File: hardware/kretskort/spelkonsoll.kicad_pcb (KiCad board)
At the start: 2 copper layers, 176.6 x 56.6 mm, 19 parts, among them J1 USB_C_Receptacle_USB2.0, SW1 SW_Push, SW10 SW_Push, SW11 SW_Push, SW12 SW_Push, SW2 SW_Push, SW3 SW_Push, SW4 SW_Push, SW5 SW_Push, SW6 SW_Push, SW7 SW_Push, SW8 SW_Push, SW9 SW_Push, U1 BQ24202DGN, U2 ESP32-DEVKITC-32D, U3 ILI9488

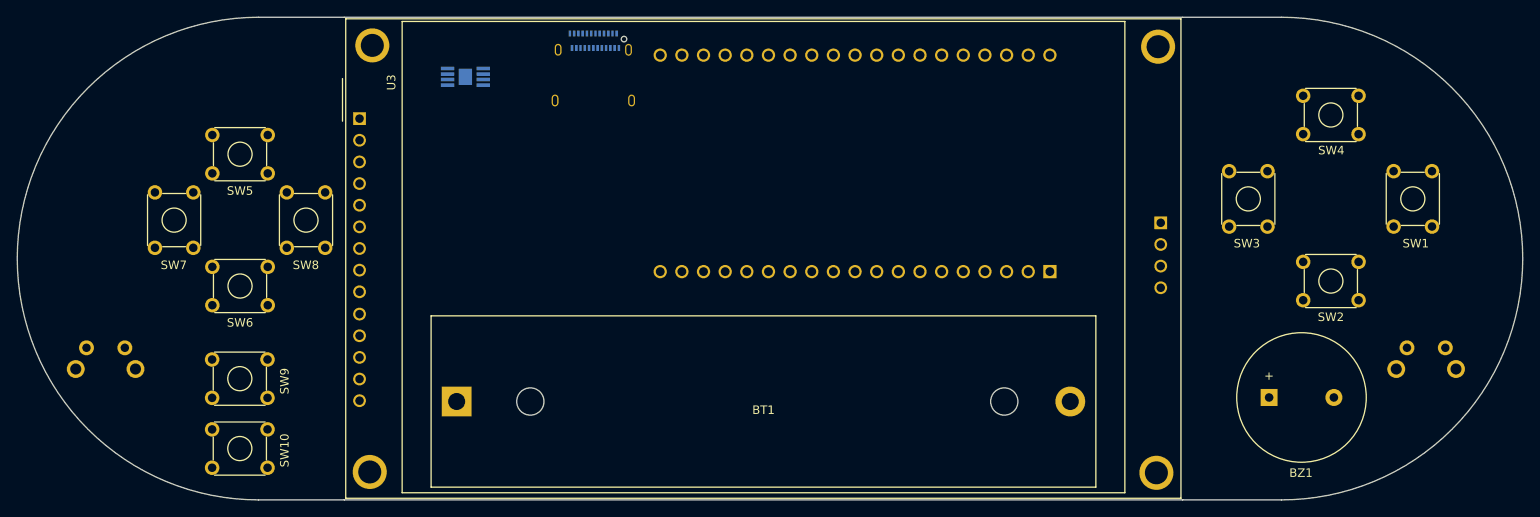
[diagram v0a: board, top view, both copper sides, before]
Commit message: lol glemte å lagre
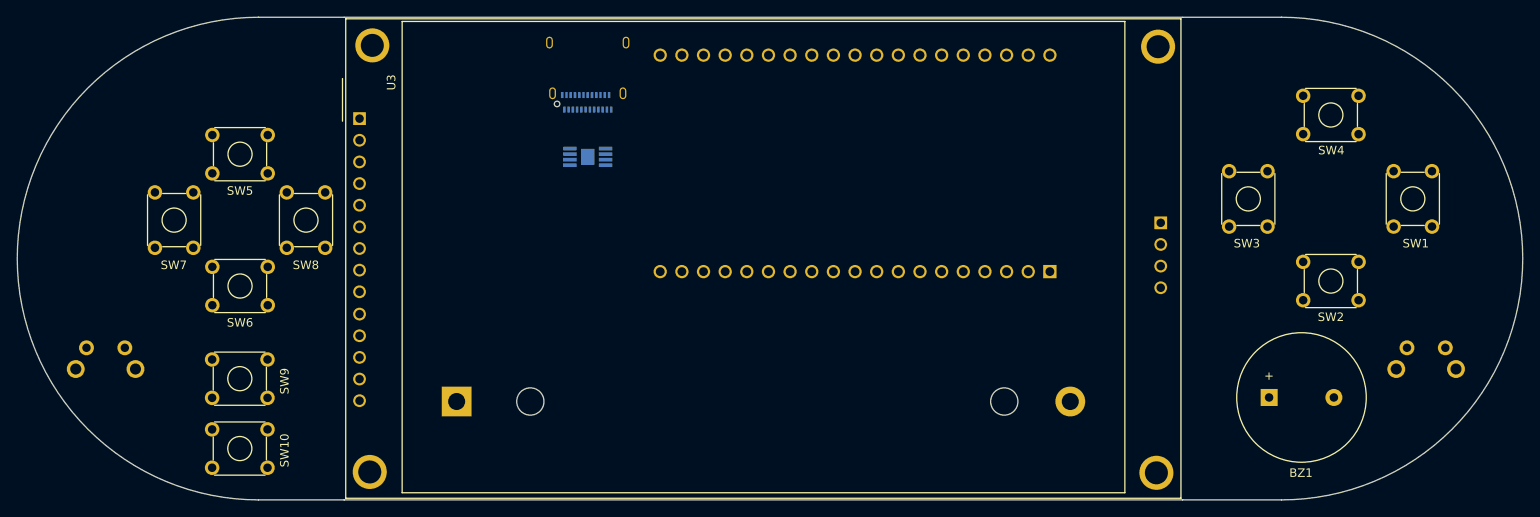
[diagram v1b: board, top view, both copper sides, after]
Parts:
- BT1: moved to B.Cu
- moved U1 17.2 mm to (124.8, 85.6)
- moved G*** 7.73 mm to (109.2, 92.7)
- moved J1 1.29 mm to (124.8, 75.0), turned to 0 degrees
